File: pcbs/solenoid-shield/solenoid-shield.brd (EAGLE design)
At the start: 54 x 58.4 mm, 75 parts, among them IC1 PCF8574TS, Q1 35A/25V/8.5mΩ, Q2 220mA/50V/3.5Ω, Q3 220mA/50V/3.5Ω, Q4 220mA/50V/3.5Ω, Q5 220mA/50V/3.5Ω, Q6 220mA/50V/3.5Ω, Q7 220mA/50V/3.5Ω, Q8 220mA/50V/3.5Ω, Q9 220mA/50V/3.5Ω, X1 2520-

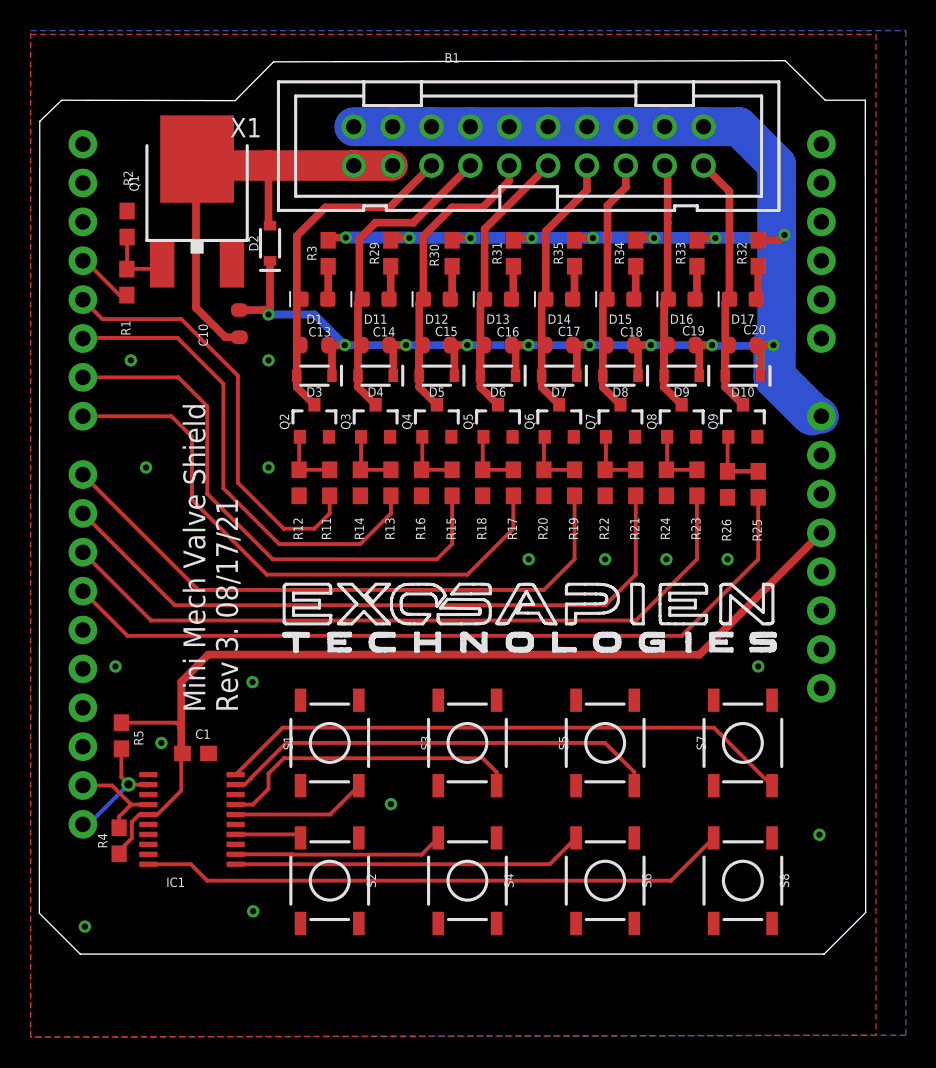
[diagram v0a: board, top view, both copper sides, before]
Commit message: Update boards to latest
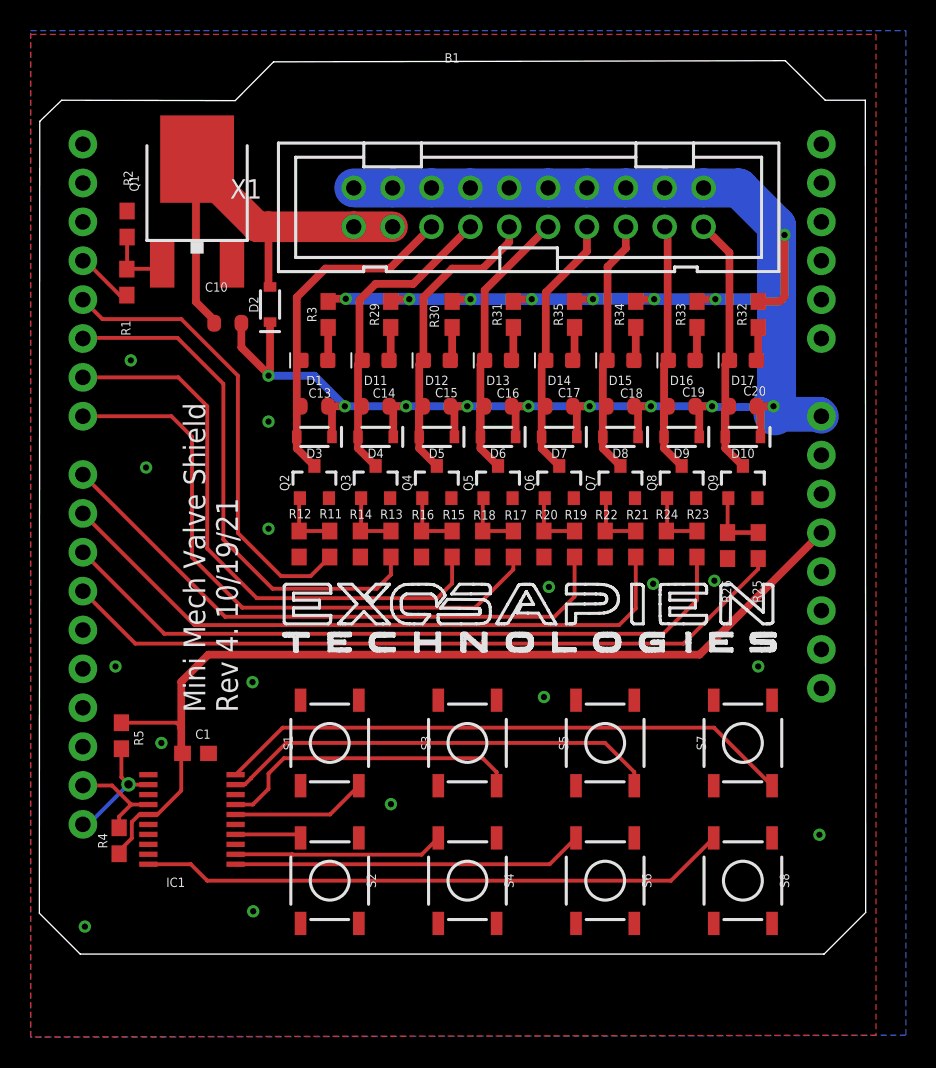
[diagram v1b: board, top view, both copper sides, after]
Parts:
- moved C13 4.00 mm to (18.0, 38.0)
- moved C14 4.00 mm to (22.0, 38.0)
- moved C15 4.00 mm to (26.0, 38.0)
- moved C16 4.00 mm to (30.0, 38.0)
- moved C17 4.00 mm to (34.0, 38.0)
- moved C18 4.00 mm to (38.0, 38.0)
- moved C19 4.00 mm to (42.0, 38.0)
- moved C20 4.00 mm to (46.0, 38.0)
- moved D1 4.00 mm to (18.0, 41.0)
- moved D10 4.00 mm to (46.0, 36.0)
- moved D11 4.00 mm to (22.0, 41.0)
- moved D12 4.00 mm to (26.0, 41.0)
- moved D13 4.00 mm to (30.0, 41.0)
- moved D14 4.00 mm to (34.0, 41.0)
- moved D15 4.00 mm to (38.0, 41.0)
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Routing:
- net VIN: track 151.9 -> 166.9 mm
- net ROUTERHIP: track 51.5 -> 48.3 mm
- net LOHIP: track 31.7 -> 34.4 mm
- net LOKNEE: track 28.0 -> 30.2 mm
- net ROUTERKNEE: track 47.8 -> 46.1 mm
- net LINKNEE: track 36.0 -> 37.7 mm
- net RINNERHIP: track 44.6 -> 43.0 mm
- net LINNERHIP: track 38.2 -> 39.8 mm
- net RINNERKNEE: track 40.2 -> 39.1 mm
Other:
- board text added: "Mini Mech Valve Shield Rev 4. 10/19/21"
- board text removed: "Mini Mech Valve Shield Rev 3. 08/17/21"
